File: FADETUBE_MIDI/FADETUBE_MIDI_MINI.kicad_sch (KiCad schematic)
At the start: 15 parts, among them J1_DECK_A1 B8B-PH-K-S, J2_DECK_B1 B8B-PH-K-S

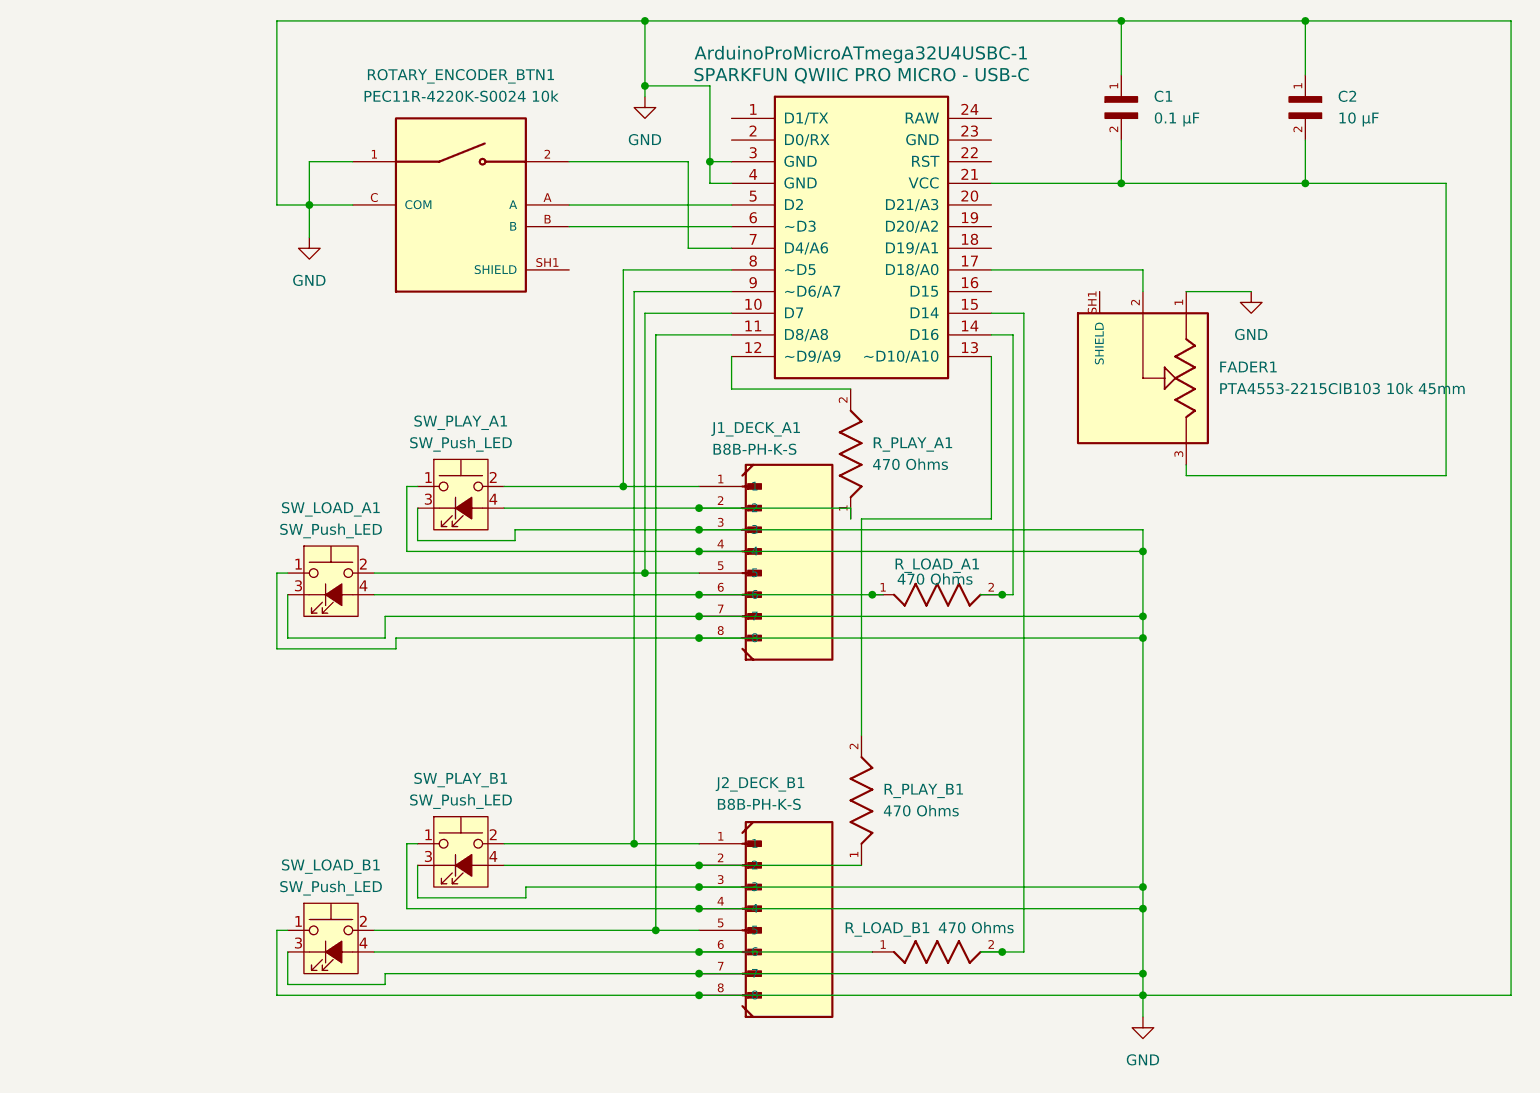
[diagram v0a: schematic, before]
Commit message: new updates
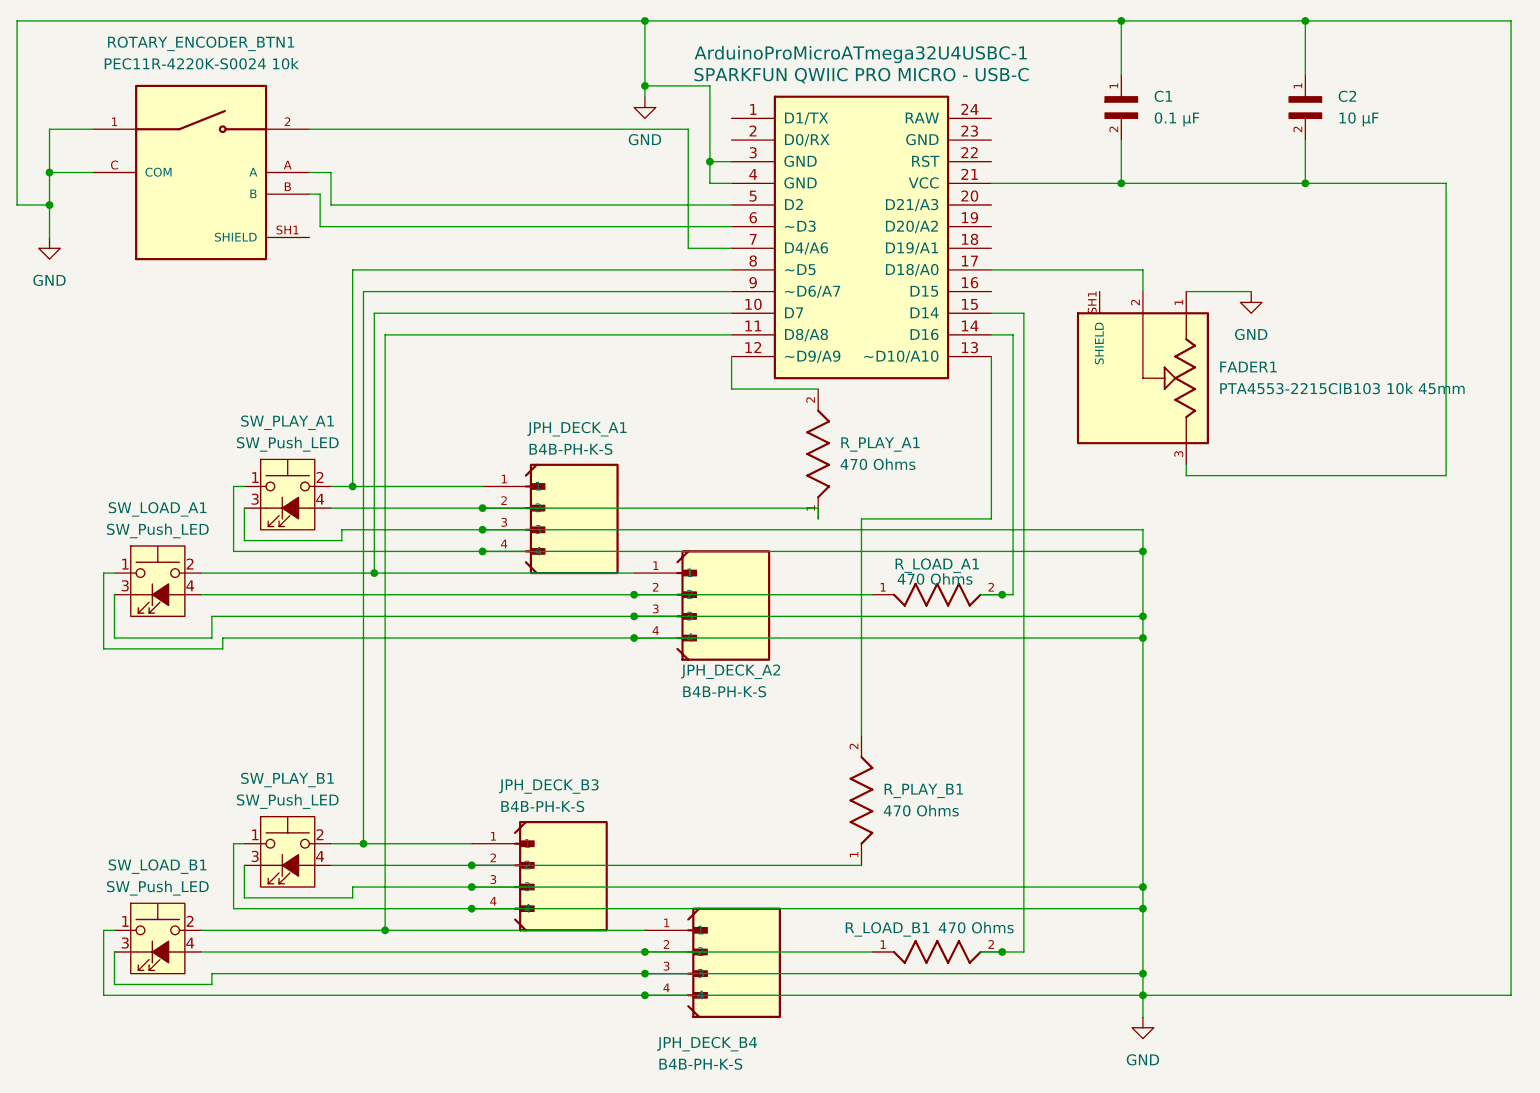
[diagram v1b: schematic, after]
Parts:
- removed J1_DECK_A1, J2_DECK_B1: B8B-PH-K-S, FADETUBE_LIBRARY:JST_B8B-PH-K-S, symbol FADETUBE_LIBRARY:B8B-PH-K-S
- added JPH_DECK_A1, JPH_DECK_A2, JPH_DECK_B3, JPH_DECK_B4: B4B-PH-K-S, FADETUBE_LIBRARY:JST_B4B-PH-K-S, symbol FADETUBE_LIBRARY:B4B-PH-K-S
- C1: footprint FADETUBE_LIBRARY:CAPC1608X90 -> Capacitor_THT:C_Disc_D3.0mm_W1.6mm_P2.50mm
- C2: footprint FADETUBE_LIBRARY:CAPC2012X88N -> Capacitor_THT:CP_Radial_D5.0mm_P2.00mm
- R_LOAD_A1, R_LOAD_B1, R_PLAY_A1, R_PLAY_B1: footprint FADETUBE_LIBRARY:RESC1608X55 -> Resistor_THT:R_Axial_DIN0207_L6.3mm_D2.5mm_P7.62mm_Horizontal
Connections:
- net GND: now also JPH_DECK_A1.3, JPH_DECK_A1.4, JPH_DECK_A2.3, JPH_DECK_A2.4, JPH_DECK_B3.3, JPH_DECK_B3.4, JPH_DECK_B4.3, JPH_DECK_B4.4
- net at ArduinoProMicroATmega32U4USBC-1.11 (D8/A8), SW_LOAD_B1.2: now also JPH_DECK_B4.1
- net at R_LOAD_B1.1, SW_LOAD_B1.4 (A): now also JPH_DECK_B4.2
- net at ArduinoProMicroATmega32U4USBC-1.8 (~D5), SW_PLAY_A1.2: now also JPH_DECK_A1.1
- net at R_PLAY_A1.1, SW_PLAY_A1.4 (A): now also JPH_DECK_A1.2
- net at ArduinoProMicroATmega32U4USBC-1.10 (D7), SW_LOAD_A1.2: now also JPH_DECK_A2.1
- net at R_LOAD_A1.1, SW_LOAD_A1.4 (A): now also JPH_DECK_A2.2
- net at ArduinoProMicroATmega32U4USBC-1.9 (~D6/A7), SW_PLAY_B1.2: now also JPH_DECK_B3.1
- net at R_PLAY_B1.1, SW_PLAY_B1.4 (A): now also JPH_DECK_B3.2
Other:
- moved on the sheet: ROTARY_ENCODER_BTN1, R_PLAY_A1, SW_LOAD_A1, SW_LOAD_B1, SW_PLAY_A1, SW_PLAY_B1
